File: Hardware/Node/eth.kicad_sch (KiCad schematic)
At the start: 1 part, among them U2 LAN8710A-EZC

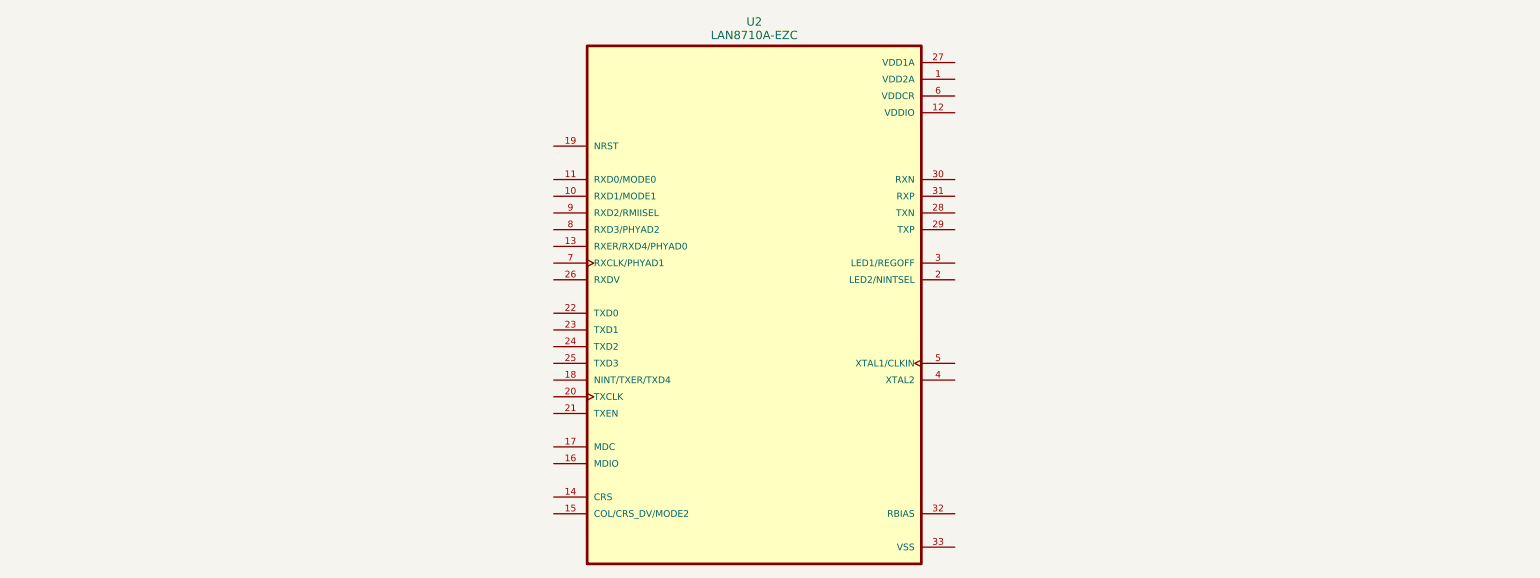
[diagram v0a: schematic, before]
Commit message: Updated schematic
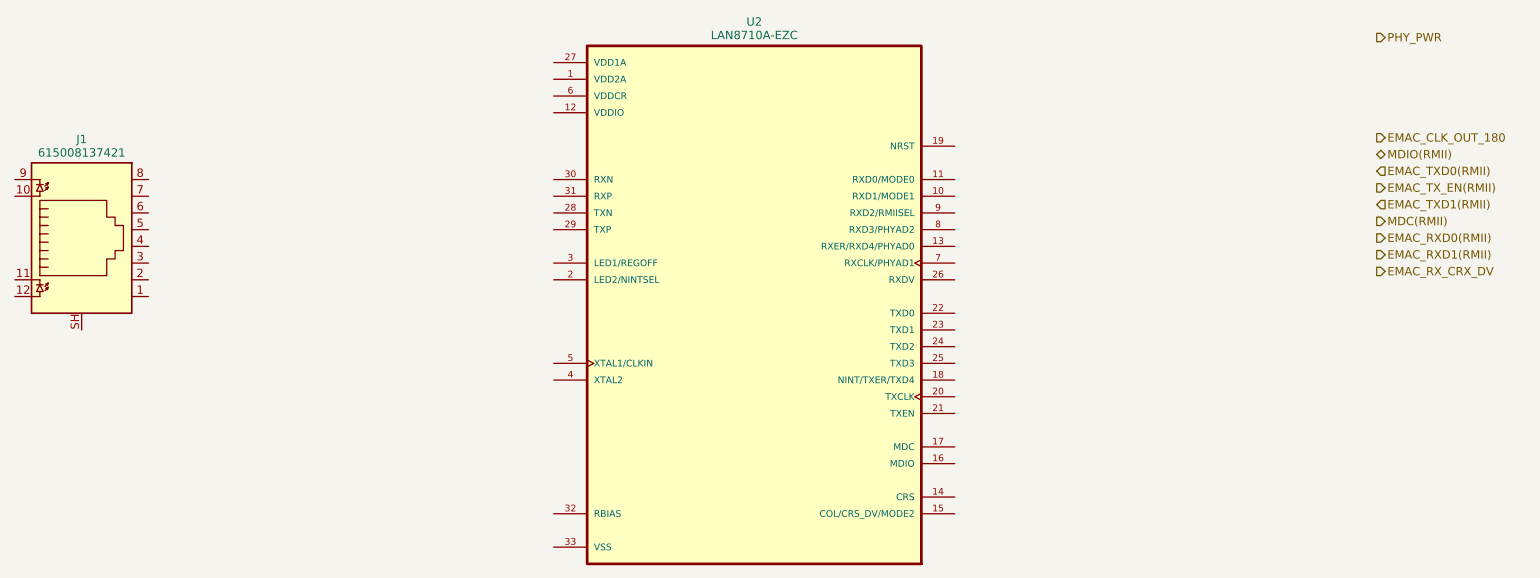
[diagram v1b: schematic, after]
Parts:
- added J1: 615008137421, manul_tech:615008137421, symbol manul_tech:615008137421
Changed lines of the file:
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@@
 (kicad_sch (version 20230121) (generator eeschema)
   (paper "A4")
-  (symbol (lib_id "manul_tech:LAN8710A-EZC") (at 139.7 89.535 0) (unit 1)
+  (hierarchical_label "EMAC_TXD0(RMII)" (shape input) (at 234.315 67.945 0) (fields_autoplaced)
+    (effects (font (size 1.27 1.27)) (justify left))
+  )
+  (hierarchical_label "EMAC_TX_EN(RMII)" (shape output) (at 234.315 70.485 0) (fields_autoplaced)
+    (effects (font (size 1.27 1.27)) (justify left))
+  )
+  (hierarchical_label "EMAC_CLK_OUT_180" (shape output) (at 234.315 62.865 0) (fields_autoplaced)
+    (effects (font (size 1.27 1.27)) (justify left))
+  )
+  (hierarchical_label "EMAC_RX_CRX_DV" (shape output) (at 234.315 83.185 0) (fields_autoplaced)
+    (effects (font (size 1.27 1.27)) (justify left))
+  )
+  (hierarchical_label "EMAC_TXD1(RMII)" (shape input) (at 234.315 73.025 0) (fields_autoplaced)
+    (effects (font (size 1.27 1.27)) (justify left))
+  )
+  (hierarchical_label "MDIO(RMII)" (shape bidirectional) (at 234.315 65.405 0) (fields_autoplaced)
+    (effects (font (size 1.27 1.27)) (justify left))
+  )
+  (hierarchical_label "MDC(RMII)" (shape output) (at 234.315 75.565 0) (fields_autoplaced)
+    (effects (font (size 1.27 1.27)) (justify left))
+  )
+  (hierarchical_label "EMAC_RXD1(RMII)" (shape output) (at 234.315 80.645 0) (fields_autoplaced)
+    (effects (font (size 1.27 1.27)) (justify left))
+  )
+  (hierarchical_label "PHY_PWR" (shape output) (at 234.315 47.625 0) (fields_autoplaced)
+    (effects (font (size 1.27 1.27)) (justify left))
+  )
+  (hierarchical_label "EMAC_RXD0(RMII)" (shape output) (at 234.315 78.105 0) (fields_autoplaced)
+    (effects (font (size 1.27 1.27)) (justify left))
+  )
+  (symbol (lib_id "manul_tech:615008137421") (at 37.465 79.375 0) (unit 1)
     (in_bom yes) (on_board yes) (dnp no) (fields_autoplaced)
+    (property "Reference" "J1" (at 37.465 63.095 0)
+      (effects (font (size 1.27 1.27)))
+    )
+    (property "Value" "615008137421" (at 37.465 65.143 0)
+      (effects (font (size 1.27 1.27)))
+    )
+    (property "Footprint" "manul_tech:615008137421" (at 37.465 78.74 90)
+      (effects (font (size 1.27 1.27)) hide)
+    )
+    (property "Datasheet" "~" (at 37.465 78.74 90)
+      (effects (font (size 1.27 1.27)) hide)
+    )
+    (pin "1")
+    (pin "10")
+    (pin "11")
+    (pin "12")
+    (pin "2")
+    (pin "3")
+    (pin "4")
+    (pin "5")
+    (pin "6")
+    (pin "7")
+    (pin "8")
+    (pin "9")
+    (pin "SH")
+    (instances
+      (project "Node"
+        (path "/48ecc24b-1ca1-455a-ac86-9597a620a90f/562b41a4-1da3-4adb-b342-096fc2b40a9a"
+          (reference "J1") (unit 1)
+        )
+      )
+    )
+  )
+  (symbol (lib_id "manul_tech:LAN8710A-EZC") (at 139.7 89.535 0) (mirror y) (unit 1)
+    (in_bom yes) (on_board yes) (dnp no)
     (property "Reference" "U2" (at 139.7 45.237 0)
       (effects (font (size 1.27 1.27)))
